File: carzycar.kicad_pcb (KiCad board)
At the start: 2 copper layers, 80 x 80 mm, 0 parts

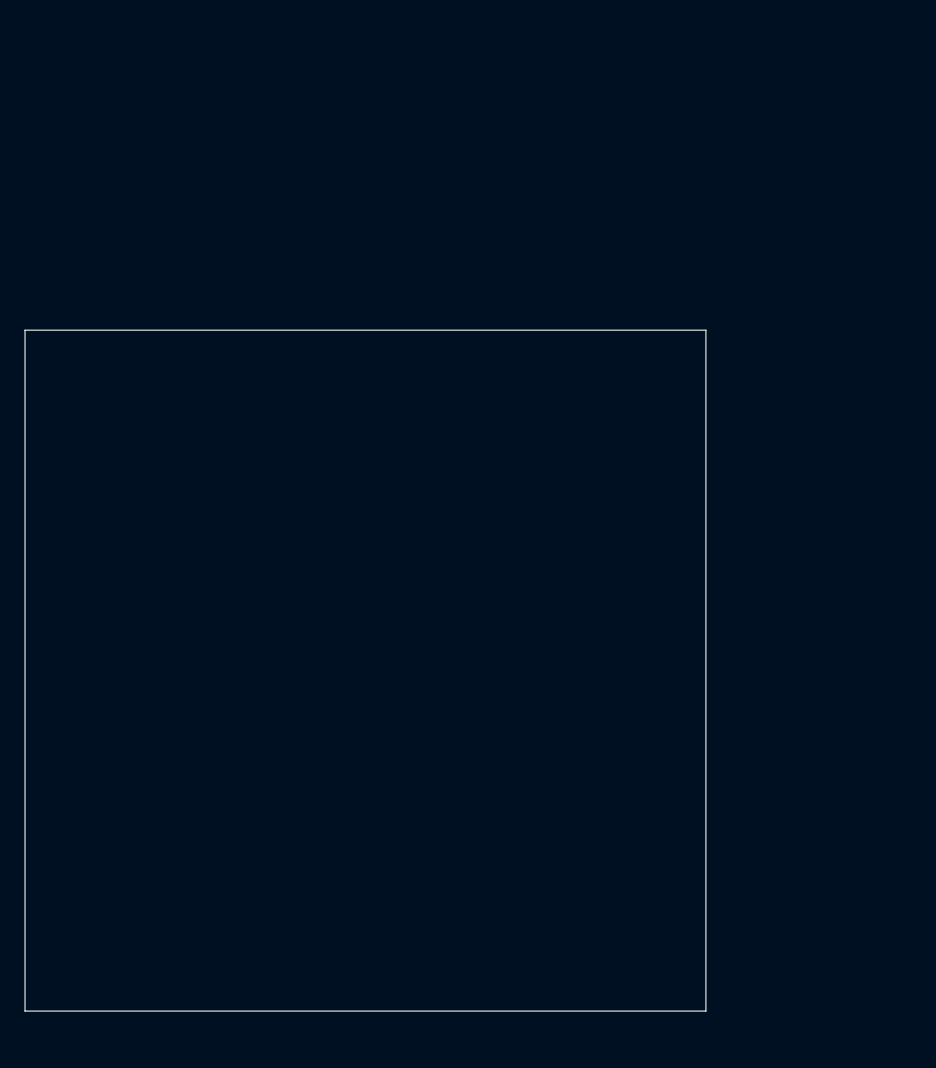
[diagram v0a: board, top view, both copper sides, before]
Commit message: update only layout missing
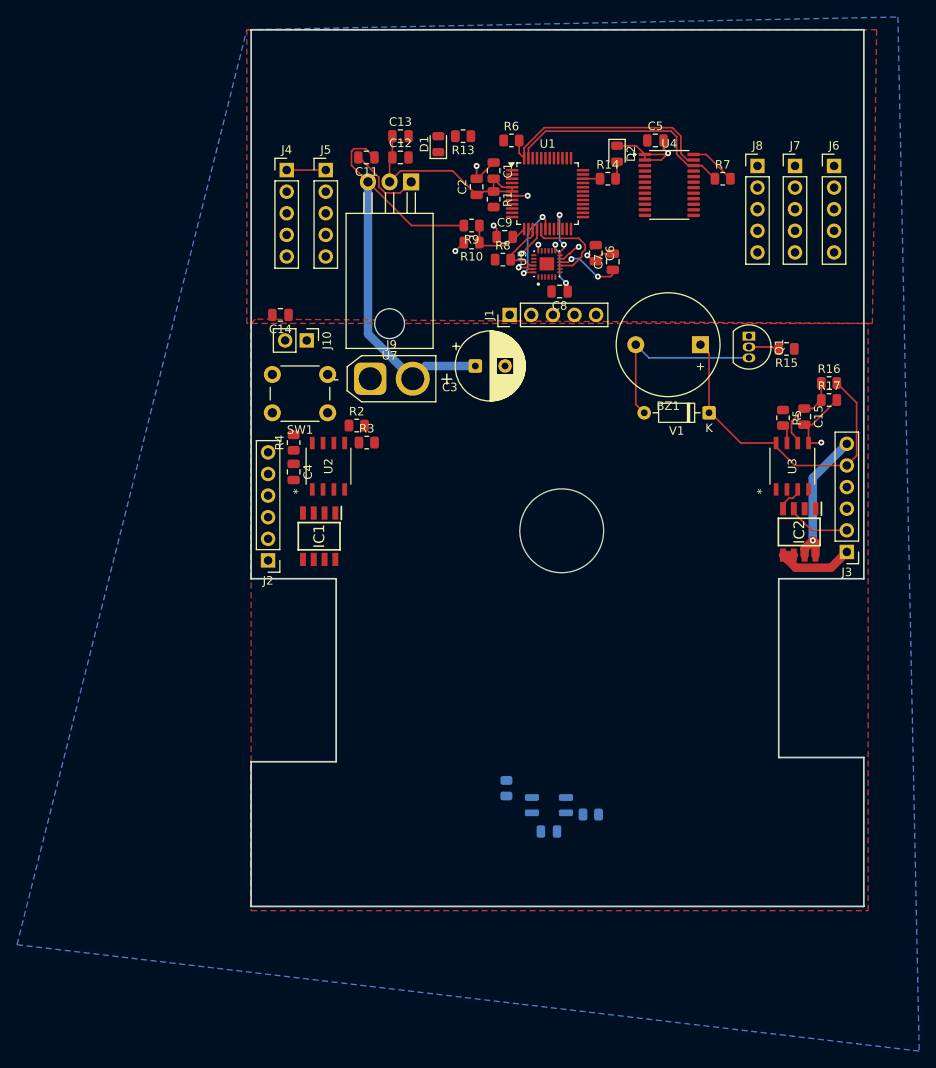
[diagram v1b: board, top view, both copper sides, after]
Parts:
- added BZ1: Buzzer, Buzzer_Beeper:Buzzer_12x9.5RM7.6, F.Cu at (151.8, 92.0)
- added C1: 100n, Capacitor_SMD:C_0805_2012Metric, F.Cu at (127.5, 71.5)
- added C10: 1n, Capacitor_SMD:C_0805_2012Metric, B.Cu at (134.0, 149.2)
- added C11: 10u, Capacitor_SMD:C_0805_2012Metric, F.Cu at (112.5, 70.0)
- added C12: 100n, Capacitor_SMD:C_0805_2012Metric, F.Cu at (116.5, 70.0)
- added C13: 10u, Capacitor_SMD:C_0805_2012Metric, F.Cu at (116.5, 67.5)
- added C14: 100n, Capacitor_SMD:C_0805_2012Metric, F.Cu at (102.5, 88.5)
- added C15: 100n, Capacitor_SMD:C_0805_2012Metric, F.Cu at (164.0, 100.5)
- added C2: 100n, Capacitor_SMD:C_0805_2012Metric, F.Cu at (125.5, 73.5)
- added C3: 470uF, Capacitor_THT:CP_Radial_D8.0mm_P3.50mm, F.Cu at (125.3, 94.5)
- added C4: 100n, Capacitor_SMD:C_0805_2012Metric, F.Cu at (104.0, 107.0)
- added C5: 100n, Capacitor_SMD:C_0805_2012Metric, F.Cu at (146.5, 68.0)
- added C6: 10n, Capacitor_SMD:C_0805_2012Metric, F.Cu at (139.5, 81.2)
- added C7: 100n, Capacitor_SMD:C_0805_2012Metric, F.Cu at (141.5, 82.2)
- added C8: 100n, Capacitor_SMD:C_0805_2012Metric, F.Cu at (135.2, 85.8)
- added C9: 100n, Capacitor_SMD:C_0805_2012Metric, F.Cu at (128.8, 79.3)
- added D1: LED, LED_SMD:LED_0805_2012Metric, F.Cu at (121.0, 68.4)
- added D2: LED, LED_SMD:LED_0805_2012Metric, F.Cu at (142.0, 69.6)
- added IC1: RZ7889, RZ7889:SOIC127P600X175-8N, F.Cu at (107.0, 114.5)
- added IC2: RZ7889, RZ7889:SOIC127P600X175-8N, F.Cu at (163.4, 114.0)
- added J1: SWD header, Connector_PinHeader_2.54mm:PinHeader_1x05_P2.54mm_Vertical, F.Cu at (129.4, 88.5)
- added J10: Conn_01x02_Socket, Connector_PinHeader_2.54mm:PinHeader_1x02_P2.54mm_Vertical, F.Cu at (105.5, 91.5)
- added J2: Conn_01x06_Pin, Connector_PinHeader_2.54mm:PinHeader_1x06_P2.54mm_Vertical, F.Cu at (101.0, 117.3)
- added J3: Conn_01x06_Pin, Connector_PinHeader_2.54mm:PinHeader_1x06_P2.54mm_Vertical, F.Cu at (169.0, 116.3)
- added J4: VL53L0X, Connector_PinHeader_2.54mm:PinHeader_1x05_P2.54mm_Vertical, F.Cu at (103.2, 71.5)
- added J5: VL53L0X, Connector_PinHeader_2.54mm:PinHeader_1x05_P2.54mm_Vertical, F.Cu at (107.8, 71.5)
- added J6: VL53L0X, Connector_PinHeader_2.54mm:PinHeader_1x05_P2.54mm_Vertical, F.Cu at (167.5, 71.0)
- added J7: VL53L0X, Connector_PinHeader_2.54mm:PinHeader_1x05_P2.54mm_Vertical, F.Cu at (162.9, 71.0)
- added J8: VL53L0X, Connector_PinHeader_2.54mm:PinHeader_1x05_P2.54mm_Vertical, F.Cu at (158.5, 71.0)
- added J9: Conn_01x02_Socket, Connector_AMASS:AMASS_XT30U-F_1x02_P5.0mm_Vertical, F.Cu at (113.0, 96.0)
- added Q1: 2N3904, Package_TO_SOT_THT:TO-92_Inline, F.Cu at (157.5, 91.0)
- added R1: 10k, Resistor_SMD:R_0805_2012Metric, F.Cu at (127.5, 74.9)
- added R10: 10k, Resistor_SMD:R_0805_2012Metric, F.Cu at (124.9, 80.0)
- added R11: 68R, Resistor_SMD:R_0805_2012Metric, B.Cu at (129.0, 144.1)
- added R12: 47k, Resistor_SMD:R_0805_2012Metric, B.Cu at (138.9, 147.2)
- added R13: 330R, Resistor_SMD:R_0805_2012Metric, F.Cu at (123.9, 67.5)
- added R14: 330R, Resistor_SMD:R_0805_2012Metric, F.Cu at (140.9, 72.5)
- added R15: 1k, Resistor_SMD:R_0805_2012Metric, F.Cu at (161.9, 92.5)
- added R16: 10k, Resistor_SMD:R_0805_2012Metric, F.Cu at (166.9, 96.5)
- added R17: 10k, Resistor_SMD:R_0805_2012Metric, F.Cu at (166.9, 98.5)
- added R2: 10k, Resistor_SMD:R_0805_2012Metric, F.Cu at (111.4, 101.5)
- added R3: 10k, Resistor_SMD:R_0805_2012Metric, F.Cu at (112.6, 103.5)
- added R4: 100R, Resistor_SMD:R_0805_2012Metric, F.Cu at (104.0, 103.5)
- added R5: 100R, Resistor_SMD:R_0805_2012Metric, F.Cu at (161.5, 100.6)
- added R6: 4k7, Resistor_SMD:R_0805_2012Metric, F.Cu at (129.6, 68.0)
- added R7: 4k7, Resistor_SMD:R_0805_2012Metric, F.Cu at (154.4, 72.5)
- added R8: 10k, Resistor_SMD:R_0805_2012Metric, F.Cu at (128.6, 82.0)
- added R9: 33k, Resistor_SMD:R_0805_2012Metric, F.Cu at (124.9, 78.0)
- added SW1: Push_Button, Button_Switch_THT:SW_PUSH_6mm, F.Cu at (108.0, 100.0)
- added U1: STM32C031C4Tx, Package_QFP:LQFP-48_7x7mm_P0.5mm, F.Cu at (133.8, 74.2)
- added U2: TMCS1100A3QDR, TMCS1100A1:SOIC8_D_TEX, F.Cu at (108.1, 106.3)
- added U3: TMCS1100A3QDR, TMCS1100A1:SOIC8_D_TEX, F.Cu at (162.6, 106.3)
- added U4: TCA9548APWR, Package_SO:TSSOP-24_4.4x7.8mm_P0.65mm, F.Cu at (148.1, 73.2)
- added U5: MPU-6500, MPU-6500:QFN40P300X300X95-25N, F.Cu at (133.8, 82.5)
- added U6: QRE1113GR, OptoDevice:OnSemi_CASE100CY, B.Cu at (134.0, 146.1)
- added U7: LD1117V33, Package_TO_SOT_THT:TO-220-3_Horizontal_TabDown, F.Cu at (117.8, 72.9)
- added V1: 1N4148, Diode_THT:D_DO-35_SOD27_P7.62mm_Horizontal, F.Cu at (152.8, 100.0)
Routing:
- net +3.3V: track 0.00 -> 78.7 mm, vias 0 -> 2
- net GND: track 0.00 -> 58.3 mm, vias 0 -> 9
- net +7.4V: track 0.00 -> 54.3 mm
- net SCL: track 0.00 -> 27.4 mm
- net SDA: track 0.00 -> 27.2 mm
- net Net-(BZ1--): track 0.00 -> 22.3 mm
- net Net-(IC2-BO_1): track 0.00 -> 17.0 mm, vias 0 -> 1
- net SDO: track 0.00 -> 10.9 mm
- net SDI: track 0.00 -> 10.3 mm, vias 0 -> 2
- net Net-(IC2-FO_1): track 0.00 -> 9.93 mm
- net Vref1: track 0.00 -> 9.39 mm
- net V_BAT: track 0.00 -> 8.22 mm
- net Net-(U5-REGOUT): track 0.00 -> 7.91 mm, vias 0 -> 2
- net CS: track 0.00 -> 7.81 mm
- net SCK: track 0.00 -> 7.55 mm, vias 0 -> 2
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- added copper zone on F.Cu, net +3.3V
- added copper zone on F.Cu, net +7.4V
- added copper zone on B.Cu, net GND
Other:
- board size 80 x 80 mm -> 72 x 103 mm
